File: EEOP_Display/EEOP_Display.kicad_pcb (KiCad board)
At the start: 2 copper layers, 2 parts, among them J1 Conn_01x32, J2 Conn_01x32

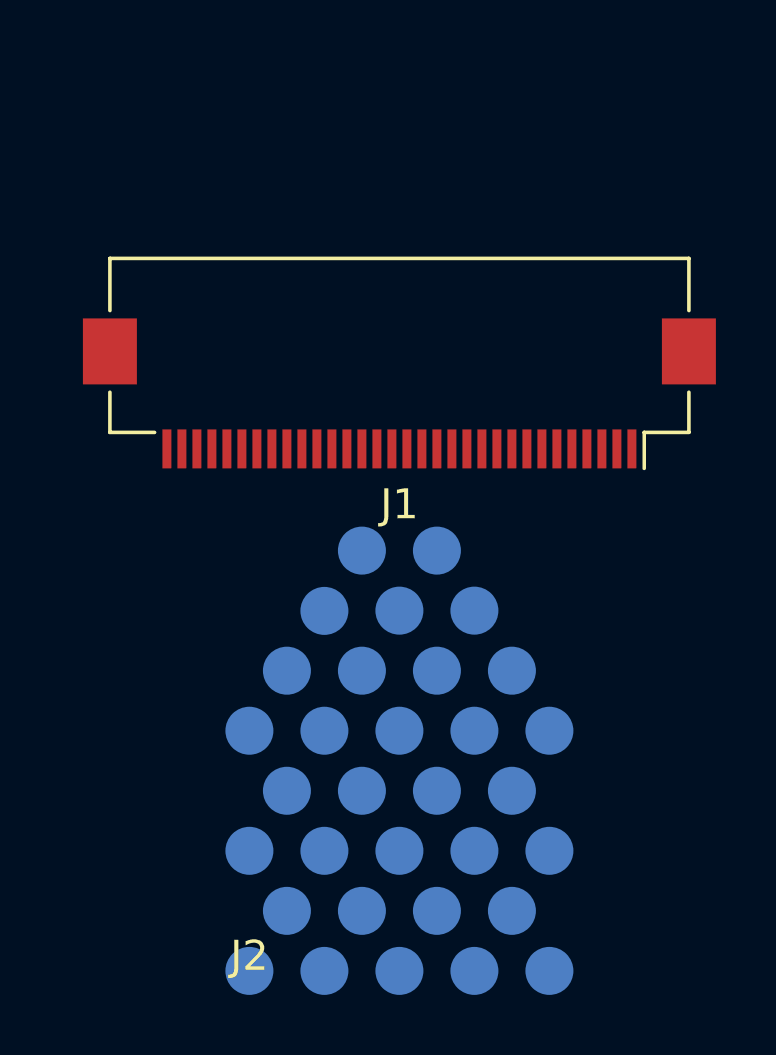
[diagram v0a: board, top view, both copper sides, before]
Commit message: Finished EEOP PCB
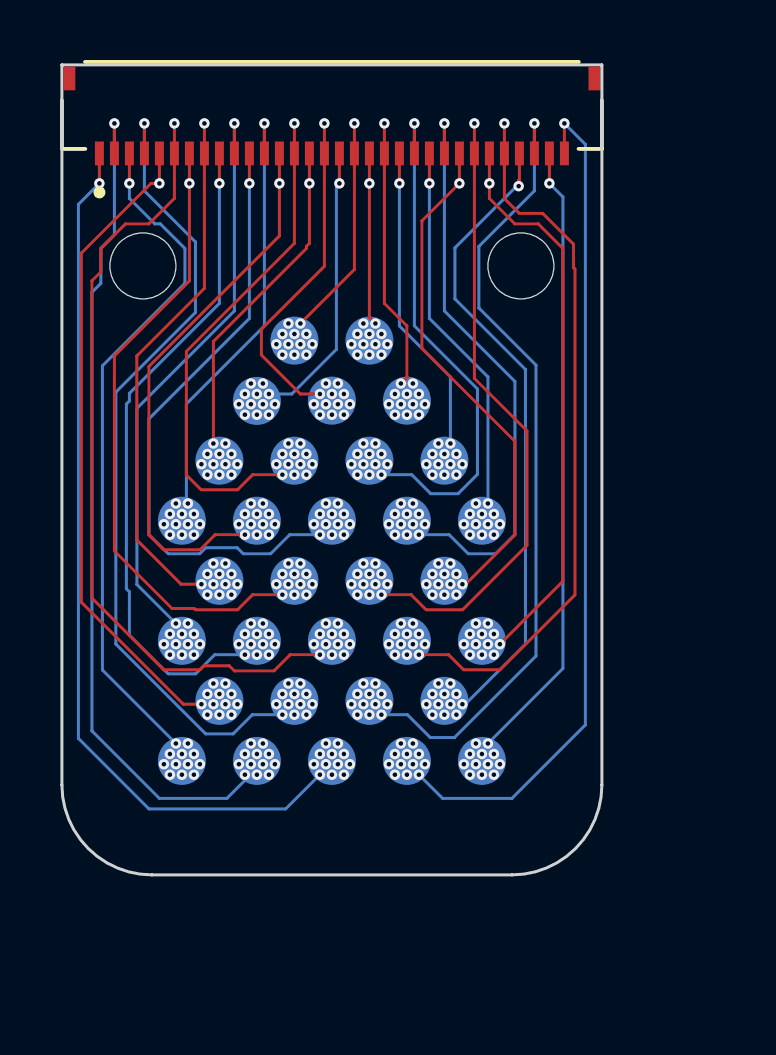
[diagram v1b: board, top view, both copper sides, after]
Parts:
- added REF**: MountingHole_2.2mm_M2, MountingHole:MountingHole_2.2mm_M2, F.Cu at (41.3, 23.5)
- added REF**: MountingHole_2.2mm_M2, MountingHole:MountingHole_2.2mm_M2, F.Cu at (28.7, 23.5)
- J1: value Conn_01x32 -> FH34SRJ-32S-0.5SH_50_; footprint Connector_FFC-FPC:Hirose_FH12-32S-0.5SH_1x32-1MP_P0.50mm_Horizontal -> Touchpoint:HRS_FH34SRJ-32S-0.5SH_50_
- moved J1 9.52 mm to (35.0, 18.5)
- moved J2 7.35 mm to (30.0, 40.0)
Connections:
- J1 pad 1: /E32 -> /E1
- J1 pad 10: /E23 -> /E10
- J1 pad 11: /E22 -> /E11
- J1 pad 12: /E21 -> /E12
- J1 pad 13: /E20 -> /E13
- J1 pad 14: /E19 -> /E14
- J1 pad 15: /E18 -> /E15
- J1 pad 16: /E17 -> /E16
- J1 pad 17: /E16 -> /E17
- J1 pad 18: /E15 -> /E18
- J1 pad 19: /E14 -> /E19
- J1 pad 2: /E31 -> /E2
- J1 pad 20: /E13 -> /E20
- J1 pad 21: /E12 -> /E21
- J1 pad 22: /E11 -> /E22
- J1 pad 23: /E10 -> /E23
- J1 pad 24: /E9 -> /E24
- J1 pad 25: /E8 -> /E25
- J1 pad 26: /E7 -> /E26
- J1 pad 27: /E6 -> /E27
- J1 pad 28: /E5 -> /E28
- J1 pad 29: /E4 -> /E29
- J1 pad 3: /E30 -> /E3
- J1 pad 30: /E3 -> /E30
- J1 pad 31: /E2 -> /E31
- J1 pad 32: /E1 -> /E32
- J1 pad 4: /E29 -> /E4
- J1 pad 5: /E28 -> /E5
- J1 pad 6: /E27 -> /E6
- J1 pad 7: /E26 -> /E7
- J1 pad 8: /E25 -> /E8
- J1 pad 9: /E24 -> /E9
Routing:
- net /E1: track 0.00 -> 29.3 mm, vias 0 -> 13
- net /E32: track 0.00 -> 28.2 mm, vias 0 -> 13
- net /E2: track 0.00 -> 28.0 mm, vias 0 -> 13
- net /E4: track 0.00 -> 27.2 mm, vias 0 -> 13
- net /E30: track 0.00 -> 26.9 mm, vias 0 -> 13
- net /E6: track 0.00 -> 26.4 mm, vias 0 -> 13
- net /E28: track 0.00 -> 23.6 mm, vias 0 -> 13
- net /E3: track 0.00 -> 22.7 mm, vias 0 -> 13
- net /E9: track 0.00 -> 22.0 mm, vias 0 -> 13
- net /E5: track 0.00 -> 21.6 mm, vias 0 -> 13
- net /E29: track 0.00 -> 21.2 mm, vias 0 -> 13
- net /E7: track 0.00 -> 20.9 mm, vias 0 -> 13
- net /E31: track 0.00 -> 20.9 mm, vias 0 -> 13
- net /E26: track 0.00 -> 20.7 mm, vias 0 -> 13
- net /E11: track 0.00 -> 20.5 mm, vias 0 -> 13
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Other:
- board outline added: 18 x 27 mm
